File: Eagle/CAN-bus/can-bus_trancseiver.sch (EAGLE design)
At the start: 10 parts

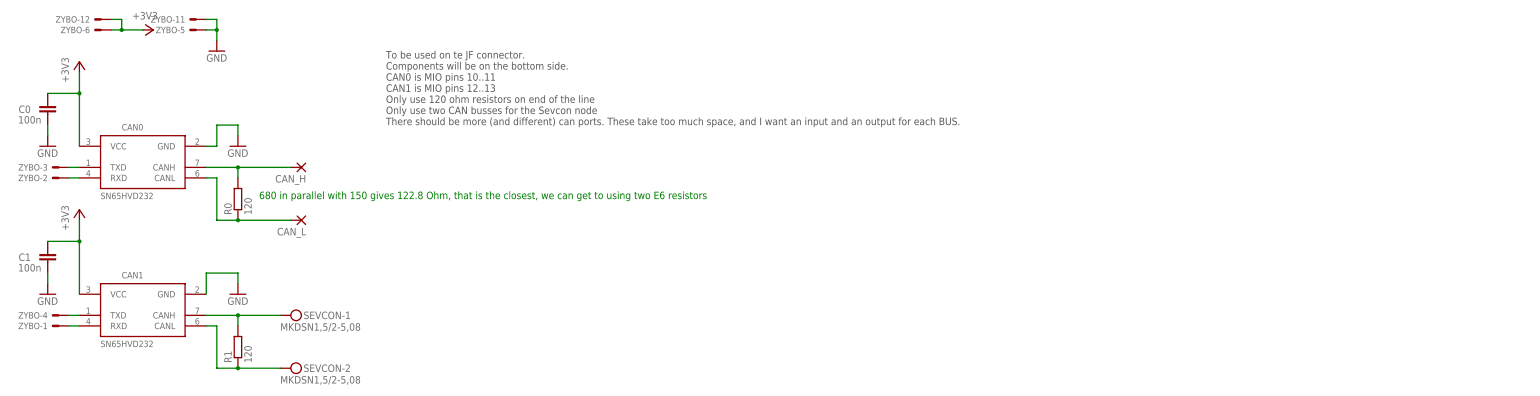
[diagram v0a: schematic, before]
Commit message: a
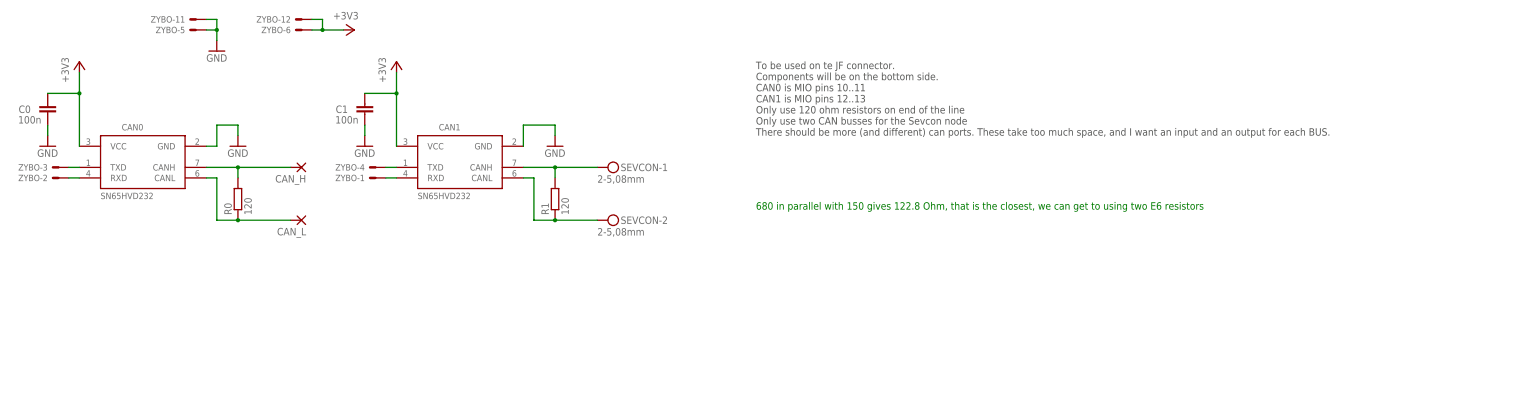
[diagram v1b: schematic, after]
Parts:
- SEVCON: value MKDSN1,5/2-5,08 -> 2-5,08mm
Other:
- moved on the sheet: C1, CAN1, R1, SEVCON-1, SEVCON-2, ZYBO-1, ZYBO-12, ZYBO-4, ZYBO-6
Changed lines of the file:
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@@
 <part name="+3V3" library="supply1" deviceset="+3V3" device=""/>
 <part name="GND3" library="supply1" deviceset="GND" device=""/>
-<part name="SEVCON" library="con-phoenix-508" deviceset="MKDSN1,5/2-5,08" device=""/>
+<part name="SEVCON" library="con-phoenix-508" deviceset="MKDSN1,5/2-5,08" device="" value="2-5,08mm"/>
 <part name="R0" library="rcl" deviceset="R-EU_" device="R0805" value="120"/>
 <part name="R1" library="rcl" deviceset="R-EU_" device="R0805" value="120"/>
@@
 <sheet>
 <plain>
-<text x="38.1" y="73.66" size="1.778" layer="97">To be used on te JF connector.
+<text x="127" y="71.12" size="1.778" layer="97">To be used on te JF connector.
 Components will be on the bottom side.
 CAN0 is MIO pins 10..11
@@
 Only use two CAN busses for the Sevcon node
 There should be more (and different) can ports. These take too much space, and I want an input and an output for each BUS.</text>
-<text x="7.62" y="55.88" size="1.778" layer="91">680 in parallel with 150 gives 122.8 Ohm, that is the closest, we can get to using two E6 resistors</text>
+<text x="127" y="53.34" size="1.778" layer="91">680 in parallel with 150 gives 122.8 Ohm, that is the closest, we can get to using two E6 resistors</text>
 </plain>
 <instances>
-<instance part="CAN1" gate="G$1" x="-20.32" y="30.48"/>
-<instance part="+3V1" gate="G$1" x="-17.78" y="96.52" rot="R270"/>
-<instance part="+3V2" gate="G$1" x="-35.56" y="53.34"/>
-<instance part="GND1" gate="1" x="2.54" y="33.02"/>
+<instance part="CAN1" gate="G$1" x="55.88" y="66.04"/>
+<instance part="+3V1" gate="G$1" x="30.48" y="96.52" rot="R270"/>
+<instance part="+3V2" gate="G$1" x="40.64" y="88.9"/>
+<instance part="GND1" gate="1" x="78.74" y="68.58"/>
 <instance part="GND2" gate="1" x="-2.54" y="91.44"/>
 <instance part="ZYBO" gate="-2" x="-38.1" y="60.96" smashed="yes" rot="R180">
 <attribute name="NAME" x="-43.18" y="61.722" size="1.524" layer="95" rot="R180"/>
 </instance>
-<instance part="ZYBO" gate="-1" x="-38.1" y="25.4" smashed="yes" rot="R180">
-<attribute name="NAME" x="-43.18" y="26.162" size="1.524" layer="95" rot="R180"/>
+<instance part="ZYBO" gate="-1" x="38.1" y="60.96" smashed="yes" rot="R180">
+<attribute name="NAME" x="33.02" y="61.722" size="1.524" layer="95" rot="R180"/>
 </instance>
 <instance part="ZYBO" gate="-3" x="-38.1" y="63.5" smashed="yes" rot="R180">
 <attribute name="NAME" x="-43.18" y="64.262" size="1.524" layer="95" rot="R180"/>
 </instance>
-<instance part="ZYBO" gate="-4" x="-38.1" y="27.94" smashed="yes" rot="R180">
-<attribute name="NAME" x="-43.18" y="28.702" size="1.524" layer="95" rot="R180"/>
+<instance part="ZYBO" gate="-4" x="38.1" y="63.5" smashed="yes" rot="R180">
+<attribute name="NAME" x="33.02" y="64.262" size="1.524" layer="95" rot="R180"/>
 </instance>
 <instance part="ZYBO" gate="-5" x="-5.08" y="96.52" smashed="yes" rot="R180">
 <attribute name="NAME" x="-10.16" y="97.282" size="1.524" layer="95" rot="R180"/>
 </instance>
-<instance part="ZYBO" gate="-6" x="-27.94" y="96.52" smashed="yes" rot="R180">
-<attribute name="NAME" x="-33.02" y="97.282" size="1.524" layer="95" rot="R180"/>
+<instance part="ZYBO" gate="-6" x="20.32" y="96.52" smashed="yes" rot="R180">
+<attribute name="NAME" x="15.24" y="97.282" size="1.524" layer="95" rot="R180"/>
 </instance>
 <instance part="ZYBO" gate="-11" x="-5.08" y="99.06" smashed="yes" rot="R180">
 <attribute name="NAME" x="-10.16" y="99.822" size="1.524" layer="95" rot="R180"/>
 </instance>
-<instance part="ZYBO" gate="-12" x="-27.94" y="99.06" smashed="yes" rot="R180">
-<attribute name="NAME" x="-33.02" y="99.822" size="1.524" layer="95" rot="R180"/>
+<instance part="ZYBO" gate="-12" x="20.32" y="99.06" smashed="yes" rot="R180">
+<attribute name="NAME" x="15.24" y="99.822" size="1.524" layer="95" rot="R180"/>
 </instance>
 <instance part="CAN0" gate="G$1" x="-20.32" y="66.04"/>
 <instance part="+3V3" gate="G$1" x="-35.56" y="88.9"/>
 <instance part="GND3" gate="1" x="2.54" y="68.58"/>
-<instance part="SEVCON" gate="-1" x="15.24" y="27.94"/>
-<instance part="SEVCON" gate="-2" x="15.24" y="15.24"/>
+<instance part="SEVCON" gate="-1" x="91.44" y="63.5"/>
+<instance part="SEVCON" gate="-2" x="91.44" y="50.8"/>
 <instance part="R0" gate="G$1" x="2.54" y="55.88" rot="R90"/>
-<instance part="R1" gate="G$1" x="2.54" y="20.32" rot="R90"/>
+<instance part="R1" gate="G$1" x="78.74" y="55.88" rot="R90"/>
 <instance part="C0" gate="G$1" x="-43.18" y="78.74" smashed="yes">
 <attribute name="NAME" x="-47.244" y="78.359" size="1.778" layer="95" rot="R180"/>
@@
 </instance>
 <instance part="GND4" gate="1" x="-43.18" y="68.58"/>
-<instance part="C1" gate="G$1" x="-43.18" y="43.18" smashed="yes">
-<attribute name="NAME" x="-47.244" y="42.799" size="1.778" layer="95" rot="R180"/>
-<attribute name="VALUE" x="-44.704" y="40.259" size="1.778" layer="96" rot="R180"/>
-</instance>
-<instance part="GND5" gate="1" x="-43.18" y="33.02"/>
+<instance part="C1" gate="G$1" x="33.02" y="78.74" smashed="yes">
+<attribute name="NAME" x="28.956" y="78.359" size="1.778" layer="95" rot="R180"/>
+<attribute name="VALUE" x="31.496" y="75.819" size="1.778" layer="96" rot="R180"/>
+</instance>
+<instance part="GND5" gate="1" x="33.02" y="68.58"/>
 <instance part="CAN_H" gate="P" x="17.78" y="63.5" rot="R180"/>
 <instance part="CAN_L" gate="P" x="17.78" y="50.8" rot="R180"/>
@@
 <segment>
 <pinref part="+3V1" gate="G$1" pin="+3V3"/>
-<wire x1="-20.32" y1="96.52" x2="-25.4" y2="96.52" width="0.1524" layer="91"/>
-<wire x1="-27.94" y1="99.06" x2="-25.4" y2="99.06" width="0.1524" layer="91"/>
-<wire x1="-25.4" y1="99.06" x2="-25.4" y2="96.52" width="0.1524" layer="91"/>
-<wire x1="-25.4" y1="96.52" x2="-27.94" y2="96.52" width="0.1524" layer="91"/>
-<junction x="-25.4" y="96.52"/>
+<wire x1="27.94" y1="96.52" x2="22.86" y2="96.52" width="0.1524" layer="91"/>
+<wire x1="20.32" y1="99.06" x2="22.86" y2="99.06" width="0.1524" layer="91"/>
+<wire x1="22.86" y1="99.06" x2="22.86" y2="96.52" width="0.1524" layer="91"/>
+<wire x1="22.86" y1="96.52" x2="20.32" y2="96.52" width="0.1524" layer="91"/>
+<junction x="22.86" y="96.52"/>
 <pinref part="ZYBO" gate="-12" pin="S"/>
 <pinref part="ZYBO" gate="-6" pin="S"/>
@@
 <pinref part="CAN1" gate="G$1" pin="VCC"/>
 <pinref part="+3V2" gate="G$1" pin="+3V3"/>
-<wire x1="-35.56" y1="33.02" x2="-35.56" y2="45.72" width="0.1524" layer="91"/>
+<wire x1="40.64" y1="68.58" x2="40.64" y2="81.28" width="0.1524" layer="91"/>
 <pinref part="C1" gate="G$1" pin="1"/>
-<wire x1="-35.56" y1="45.72" x2="-35.56" y2="50.8" width="0.1524" layer="91"/>
-<wire x1="-43.18" y1="45.72" x2="-35.56" y2="45.72" width="0.1524" layer="91"/>
-<junction x="-35.56" y="45.72"/>
+<wire x1="40.64" y1="81.28" x2="40.64" y2="86.36" width="0.1524" layer="91"/>
+<wire x1="33.02" y1="81.28" x2="40.64" y2="81.28" width="0.1524" layer="91"/>
+<junction x="40.64" y="81.28"/>
 </segment>
 <segment>
@@
 <segment>
 <pinref part="GND1" gate="1" pin="GND"/>
-<wire x1="2.54" y1="35.56" x2="2.54" y2="38.1" width="0.1524" layer="91"/>
-<wire x1="2.54" y1="38.1" x2="-5.08" y2="38.1" width="0.1524" layer="91"/>
+<wire x1="78.74" y1="71.12" x2="78.74" y2="73.66" width="0.1524" layer="91"/>
+<wire x1="78.74" y1="73.66" x2="71.12" y2="73.66" width="0.1524" layer="91"/>
 <pinref part="CAN1" gate="G$1" pin="GND"/>
-<wire x1="-5.08" y1="38.1" x2="-5.08" y2="33.02" width="0.1524" layer="91"/>
+<wire x1="71.12" y1="73.66" x2="71.12" y2="68.58" width="0.1524" layer="91"/>
 </segment>
 <segment>
@@
 <pinref part="C1" gate="G$1" pin="2"/>
 <pinref part="GND5" gate="1" pin="GND"/>
-<wire x1="-43.18" y1="38.1" x2="-43.18" y2="35.56" width="0.1524" layer="91"/>
+<wire x1="33.02" y1="73.66" x2="33.02" y2="71.12" width="0.1524" layer="91"/>
 </segment>
 <segment>
@@
 <pinref part="ZYBO" gate="-4" pin="S"/>
 <pinref part="CAN1" gate="G$1" pin="TXD"/>
-<wire x1="-38.1" y1="27.94" x2="-35.56" y2="27.94" width="0.1524" layer="91"/>
+<wire x1="38.1" y1="63.5" x2="40.64" y2="63.5" width="0.1524" layer="91"/>
 </segment>
 </net>
@@
 <pinref part="CAN1" gate="G$1" pin="RXD"/>
 <pinref part="ZYBO" gate="-1" pin="S"/>
-<wire x1="-35.56" y1="25.4" x2="-38.1" y2="25.4" width="0.1524" layer="91"/>
+<wire x1="40.64" y1="60.96" x2="38.1" y2="60.96" width="0.1524" layer="91"/>
 </segment>
 </net>
@@
 <pinref part="CAN1" gate="G$1" pin="CANH"/>
 <pinref part="R1" gate="G$1" pin="2"/>
-<wire x1="2.54" y1="27.94" x2="-5.08" y2="27.94" width="0.1524" layer="91"/>
-<wire x1="2.54" y1="25.4" x2="2.54" y2="27.94" width="0.1524" layer="91"/>
-<wire x1="12.7" y1="27.94" x2="2.54" y2="27.94" width="0.1524" layer="91"/>
-<junction x="2.54" y="27.94"/>
+<wire x1="78.74" y1="63.5" x2="71.12" y2="63.5" width="0.1524" layer="91"/>
+<wire x1="78.74" y1="60.96" x2="78.74" y2="63.5" width="0.1524" layer="91"/>
+<wire x1="88.9" y1="63.5" x2="78.74" y2="63.5" width="0.1524" layer="91"/>
+<junction x="78.74" y="63.5"/>
 <pinref part="SEVCON" gate="-1" pin="KL"/>
 </segment>
@@
 <pinref part="R1" gate="G$1" pin="1"/>
 <pinref part="CAN1" gate="G$1" pin="CANL"/>
-<wire x1="-5.08" y1="25.4" x2="-2.54" y2="25.4" width="0.1524" layer="91"/>
-<wire x1="-2.54" y1="25.4" x2="-2.54" y2="15.24" width="0.1524" layer="91"/>
-<wire x1="-2.54" y1="15.24" x2="2.54" y2="15.24" width="0.1524" layer="91"/>
-<wire x1="12.7" y1="15.24" x2="2.54" y2="15.24" width="0.1524" layer="91"/>
-<junction x="2.54" y="15.24"/>
+<wire x1="71.12" y1="60.96" x2="73.66" y2="60.96" width="0.1524" layer="91"/>
+<wire x1="73.66" y1="60.96" x2="73.66" y2="50.8" width="0.1524" layer="91"/>
+<wire x1="73.66" y1="50.8" x2="78.74" y2="50.8" width="0.1524" layer="91"/>
+<wire x1="88.9" y1="50.8" x2="78.74" y2="50.8" width="0.1524" layer="91"/>
+<junction x="78.74" y="50.8"/>
 <pinref part="SEVCON" gate="-2" pin="KL"/>
 </segment>
